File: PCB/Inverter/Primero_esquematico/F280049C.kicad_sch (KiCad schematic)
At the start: 39 parts, among them SW1 IT-1181-180G-G, U15 F280049CPZS, U16 TPS3823-33DBVR, Y1 ABM8GAIG-20.000MHZ-8-7Z-T3

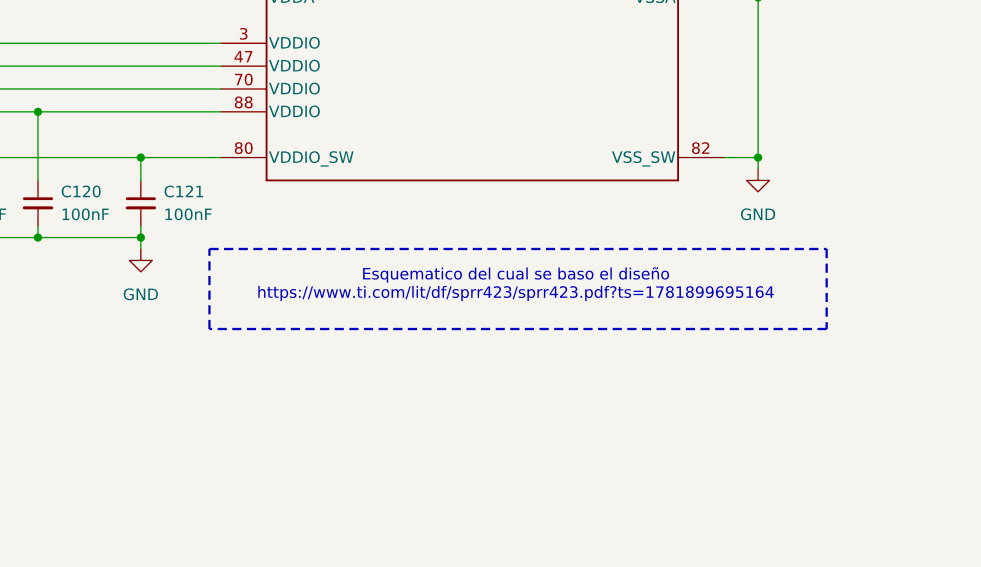
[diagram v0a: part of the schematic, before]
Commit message: a
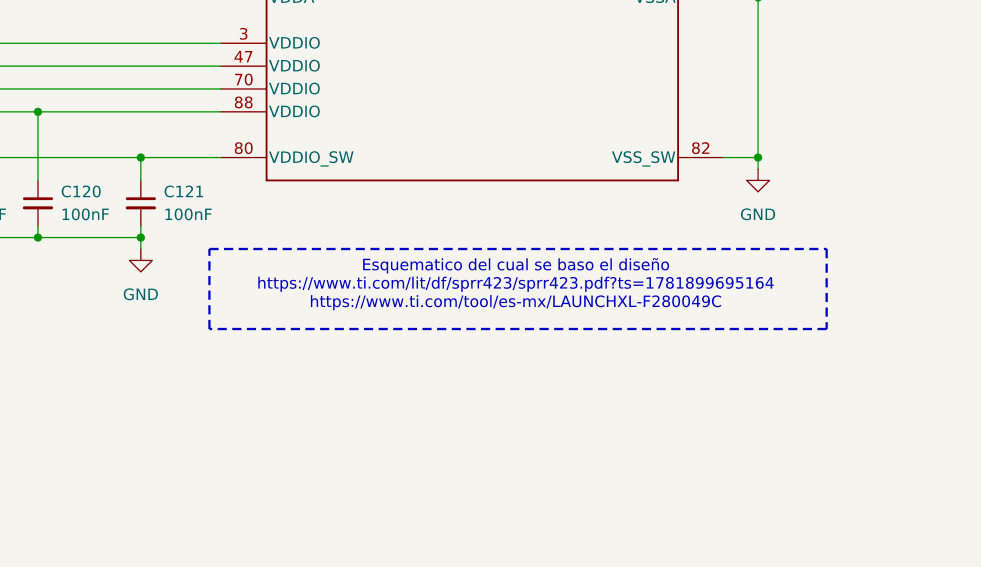
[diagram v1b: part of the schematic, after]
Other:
- note added: "Esquematico del cual se baso el diseño https://www.ti.com/lit/df/sprr423/sprr423.pdf?ts=1781899695164 https://www.ti.com/tool/es-mx/LAUNCHXL-F280049C"
- note removed: "Esquematico del cual se baso el diseño https://www.ti.com/lit/df/sprr423/sprr423.pdf?ts=1781899695164"
